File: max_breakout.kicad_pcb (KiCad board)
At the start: 4 copper layers, 51.8 x 25.9 mm, 45 parts, among them J1 Left, J2 Right, J3 AVR-JTAG-10, J4 USB_B_Micro, Q1 IRLML6402, SW1 Reset, SW2 User, SW3 User DIP Switch, SW4 ENA Switch, U1 AP7381-33SA, U2 EPM7032STC44, U3 DS1813R-5+T&R, U4 MAX40200AUK, U5 MAX40200AUK, U6 74HCT244, U7 MAX40200AUK, X1 CTX-636 50mhz

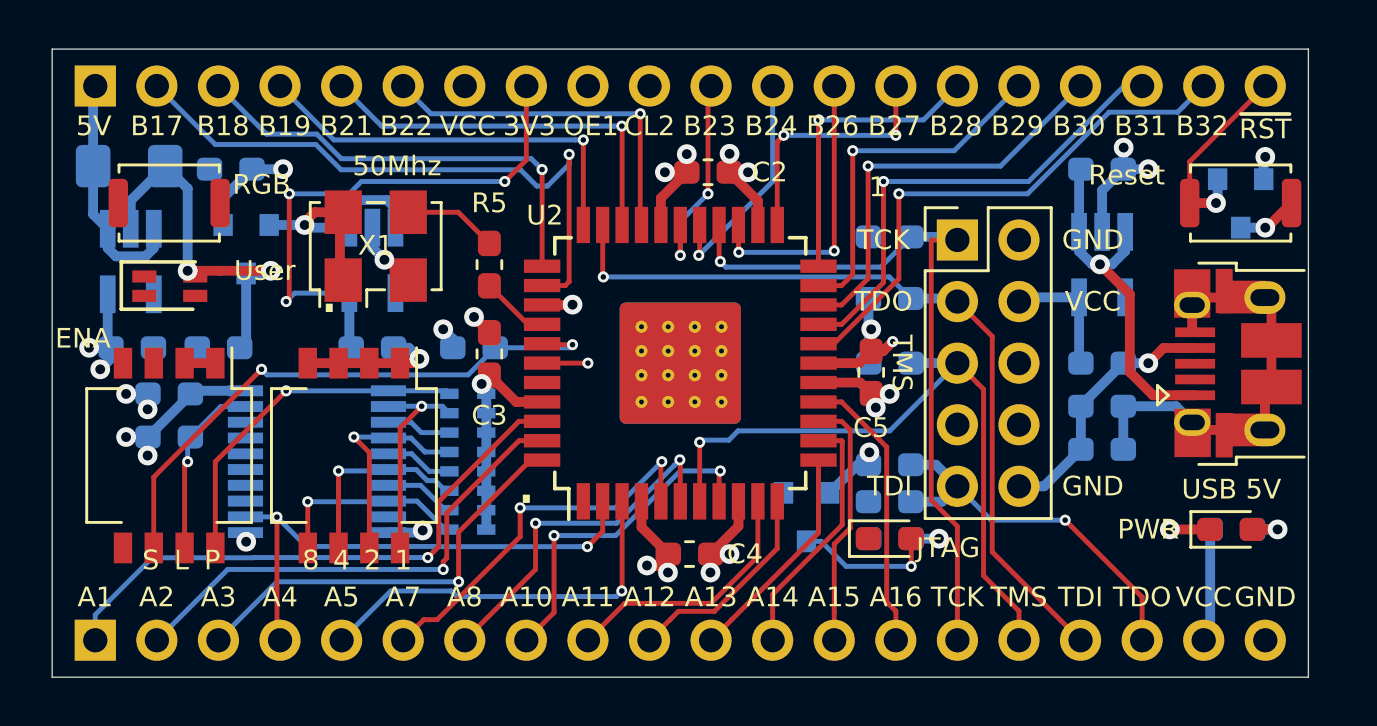
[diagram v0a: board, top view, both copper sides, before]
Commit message: more routing
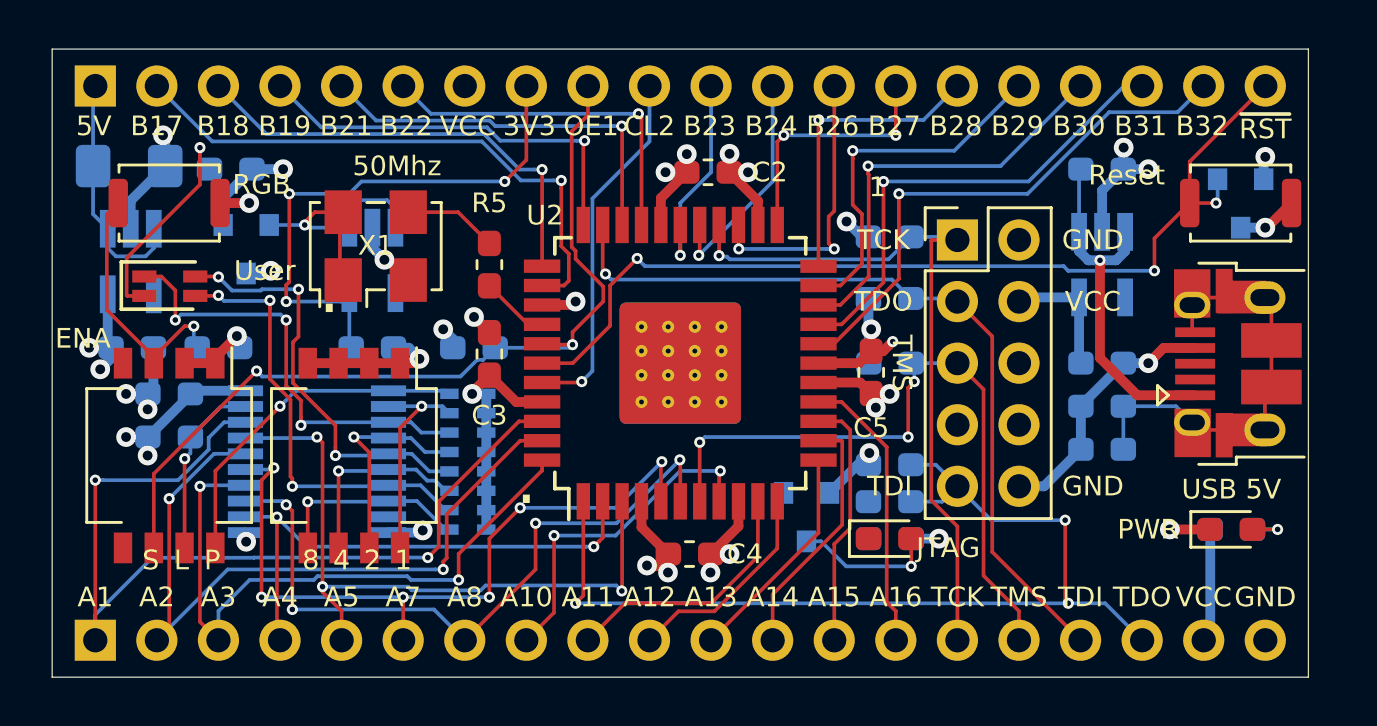
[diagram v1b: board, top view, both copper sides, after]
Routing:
- net /~RST: track 10.1 -> 39.8 mm, vias 2 -> 3
- net /TDI: track 15.8 -> 41.3 mm, vias 1 -> 3
- net /R3: track 2.69 -> 18.4 mm, vias 0 -> 3
- net /R7: track 2.94 -> 18.2 mm, vias 0 -> 3
- net /CLK2: track 0.00 -> 15.0 mm, vias 0 -> 1
- net /R5: track 2.81 -> 17.2 mm, vias 0 -> 3
- net /A7: track 16.1 -> 30.4 mm, vias 2 -> 6
- net /A1: track 23.9 -> 37.9 mm, vias 1 -> 2
- net /A8: track 14.8 -> 28.6 mm, vias 2 -> 4
- net /OE1: track 23.9 -> 36.0 mm
- net /A6: track 16.3 -> 28.1 mm, vias 1 -> 3
- net Net-(C12-Pad1): track 0.00 -> 10.7 mm, vias 0 -> 1
- net /A2: track 20.6 -> 30.5 mm, vias 1 -> 2
- net Net-(D3-Pad3): track 0.00 -> 9.13 mm, vias 0 -> 1
- net /A3: track 17.6 -> 26.7 mm, vias 1 -> 2
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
